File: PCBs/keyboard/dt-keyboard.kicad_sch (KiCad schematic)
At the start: 87 parts

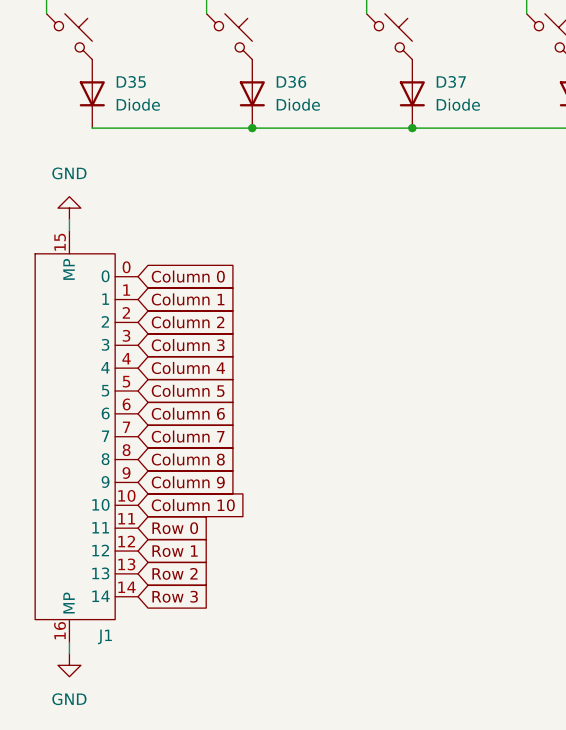
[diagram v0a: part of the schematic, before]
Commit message: Fixed Keyboard
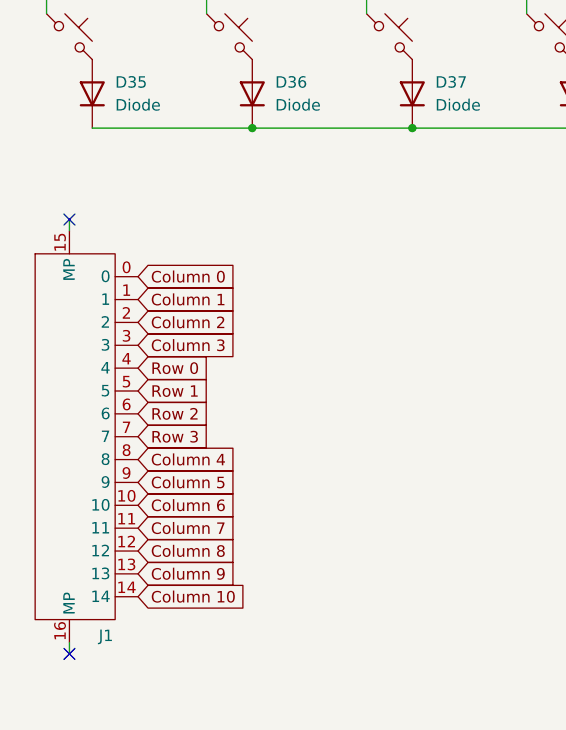
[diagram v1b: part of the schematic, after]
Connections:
- net Column 10: now also J1.14; no longer J1.10
- net Column 4: now also J1.8; no longer J1.4
- net Column 5: now also J1.9; no longer J1.5
- net Column 6: now also J1.10; no longer J1.6
- net Column 7: now also J1.11; no longer J1.7
- net Column 8: now also J1.12; no longer J1.8
- net Column 9: now also J1.13; no longer J1.9
- net Row 0: now also J1.4; no longer J1.11
- net Row 1: now also J1.5; no longer J1.12
- net Row 2: now also J1.6; no longer J1.13
- net Row 3: now also J1.7; no longer J1.14
- net GND: no longer names the net of J1.15 (MP)
- net GND: no longer J1.16 (MP)
- no-connect marks 0 -> 2
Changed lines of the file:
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@@
 		(color 0 0 0 0)
 	)
+	(no_connect
+		(at 35.56 137.16)
+	)
+	(no_connect
+		(at 35.56 185.42)
+	)
 	(wire
 		(pts
@@
 	(global_label "Row 3"
 		(shape input)
-		(at 43.18 179.07 0)
+		(at 43.18 161.29 0)
 		(fields_autoplaced yes)
 		(effects
@@
 		)
 		(property "Intersheetrefs" "${INTERSHEET_REFS}"
-			(at 52.0918 179.07 0)
+			(at 52.0918 161.29 0)
 			(effects
 				(font
@@
 	(global_label "Column 4"
 		(shape input)
-		(at 43.18 153.67 0)
+		(at 43.18 163.83 0)
 		(fields_autoplaced yes)
 		(effects
@@
 		)
 		(property "Intersheetrefs" "${INTERSHEET_REFS}"
-			(at 55.4178 153.67 0)
+			(at 55.4178 163.83 0)
 			(effects
 				(font
@@
 	(global_label "Row 2"
 		(shape input)
-		(at 43.18 176.53 0)
+		(at 43.18 158.75 0)
 		(fields_autoplaced yes)
 		(effects
@@
 		)
 		(property "Intersheetrefs" "${INTERSHEET_REFS}"
-			(at 52.0918 176.53 0)
+			(at 52.0918 158.75 0)
 			(effects
 				(font
@@
 	(global_label "Row 0"
 		(shape input)
-		(at 43.18 171.45 0)
+		(at 43.18 153.67 0)
 		(fields_autoplaced yes)
 		(effects
@@
 		)
 		(property "Intersheetrefs" "${INTERSHEET_REFS}"
-			(at 52.0918 171.45 0)
+			(at 52.0918 153.67 0)
 			(effects
 				(font
@@
 	(global_label "Column 6"
 		(shape input)
-		(at 43.18 158.75 0)
+		(at 43.18 168.91 0)
 		(fields_autoplaced yes)
 		(effects
@@
 		)
 		(property "Intersheetrefs" "${INTERSHEET_REFS}"
-			(at 55.4178 158.75 0)
+			(at 55.4178 168.91 0)
 			(effects
 				(font
@@
 	(global_label "Column 10"
 		(shape input)
-		(at 43.18 168.91 0)
+		(at 43.18 179.07 0)
 		(fields_autoplaced yes)
 		(effects
@@
 		)
 		(property "Intersheetrefs" "${INTERSHEET_REFS}"
-			(at 56.6273 168.91 0)
+			(at 56.6273 179.07 0)
 			(effects
 				(font
@@
 	(global_label "Row 1"
 		(shape input)
-		(at 43.18 173.99 0)
+		(at 43.18 156.21 0)
 		(fields_autoplaced yes)
 		(effects
@@
 		)
 		(property "Intersheetrefs" "${INTERSHEET_REFS}"
-			(at 52.0918 173.99 0)
+			(at 52.0918 156.21 0)
 			(effects
 				(font
@@
 	(global_label "Column 5"
 		(shape input)
-		(at 43.18 156.21 0)
+		(at 43.18 166.37 0)
 		(fields_autoplaced yes)
 		(effects
@@
 		)
 		(property "Intersheetrefs" "${INTERSHEET_REFS}"
-			(at 55.4178 156.21 0)
+			(at 55.4178 166.37 0)
 			(effects
 				(font
@@
 	(global_label "Column 7"
 		(shape input)
-		(at 43.18 161.29 0)
+		(at 43.18 171.45 0)
 		(fields_autoplaced yes)
 		(effects
@@
 		)
 		(property "Intersheetrefs" "${INTERSHEET_REFS}"
-			(at 55.4178 161.29 0)
+			(at 55.4178 171.45 0)
 			(effects
 				(font
@@
 	(global_label "Column 8"
 		(shape input)
-		(at 43.18 163.83 0)
+		(at 43.18 173.99 0)
 		(fields_autoplaced yes)
 		(effects
@@
 		)
 		(property "Intersheetrefs" "${INTERSHEET_REFS}"
-			(at 55.4178 163.83 0)
+			(at 55.4178 173.99 0)
 			(effects
 				(font
@@
 	(global_label "Column 9"
 		(shape input)
-		(at 43.18 166.37 0)
+		(at 43.18 176.53 0)
 		(fields_autoplaced yes)
 		(effects
@@
 		)
 		(property "Intersheetrefs" "${INTERSHEET_REFS}"
-			(at 55.4178 166.37 0)
+			(at 55.4178 176.53 0)
 			(effects
 				(font
@@
 	)
 	(symbol
-		(lib_id "power:GND")
-		(at 35.56 185.42 0)
-		(unit 1)
-		(exclude_from_sim no)
-		(in_bom yes)
-		(on_board yes)
-		(dnp no)
-		(fields_autoplaced yes)
-		(property "Reference" "#PWR01"
-			(at 35.56 191.77 0)
-			(effects
-				(font
-					(size 1.27 1.27)
-				)
-				(hide yes)
-			)
-		)
-		(property "Value" "GND"
-			(at 35.56 190.5 0)
-			(effects
-				(font
-					(size 1.27 1.27)
-				)
-			)
-		)
-		(property "Footprint" ""
-			(at 35.56 185.42 0)
-			(effects
-				(font
-					(size 1.27 1.27)
-				)
-				(hide yes)
-			)
-		)
-		(property "Datasheet" ""
-			(at 35.56 185.42 0)
-			(effects
-				(font
-					(size 1.27 1.27)
-				)
-				(hide yes)
-			)
-		)
-		(property "Description" "Power symbol creates a global label with name \"GND\" , ground"
-			(at 35.56 185.42 0)
-			(effects
-				(font
-					(size 1.27 1.27)
-				)
-				(hide yes)
-			)
-		)
-		(pin "1"
-		)
-		(instances
-			(project ""
-				(path "/a0f199ac-e5fb-4245-9c3a-54e045012dd6"
-					(reference "#PWR01")
-					(unit 1)
-				)
-			)
-		)
-	)
-	(symbol
 		(lib_id "ScottoKeebs:Placeholder_Diode")
 		(at 38.1 100.33 90)
@@
 					(unit 1)
 				)
-			)
-		)
-	)
-	(symbol
-		(lib_id "power:GND")
-		(at 35.56 137.16 180)
-		(unit 1)
-		(exclude_from_sim no)
-		(in_bom yes)
-		(on_board yes)
-		(dnp no)
-		(fields_autoplaced yes)
-		(property "Reference" "#PWR02"
-			(at 35.56 130.81 0)
-			(effects
-				(font
-					(size 1.27 1.27)
-				)
-				(hide yes)
-			)
-		)
-		(property "Value" "GND"
-			(at 35.56 132.08 0)
-			(effects
-				(font
-					(size 1.27 1.27)
-				)
-			)
-		)
-		(property "Footprint" ""
-			(at 35.56 137.16 0)
-			(effects
-				(font
-					(size 1.27 1.27)
-				)
-				(hide yes)
-			)
-		)
-		(property "Datasheet" ""
-			(at 35.56 137.16 0)
-			(effects
-				(font
-					(size 1.27 1.27)
-				)
-				(hide yes)
-			)
-		)
-		(property "Description" "Power symbol creates a global label with name \"GND\" , ground"
-			(at 35.56 137.16 0)
-			(effects
-				(font
-					(size 1.27 1.27)
-				)
-				(hide yes)
-			)
-		)
-		(pin "1"
-		)
-		(instances
-			(project "dt-keyboard"
-				(path "/a0f199ac-e5fb-4245-9c3a-54e045012dd6"
-					(reference "#PWR02")
-					(unit 1)
-				)
